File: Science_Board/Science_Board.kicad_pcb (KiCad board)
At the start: 2 copper layers, 217 x 149.5 mm, 141 parts, among them IC1 TCKE603RA, IC2 TCKE603RA, IC3 TCKE603RM, J1 Conn_01x02, J10 Conn_01x02, J11 Conn_01x03, J12 Conn_01x03, J13 Conn_01x03, J14 Conn_01x03, J15 Conn_01x03, J16 Conn_01x03, J17 Conn_01x03, J18 Conn_01x03, J19 Conn_01x02, J2 RJ45_LED_Shielded, J20 Molex_Megafit_02, J21 Molex_Megafit_02, J22 Molex_Megafit_02, J23 Conn_01x02, J3 Molex_Megafit_02, J4 Molex_Megafit_02, J5 Conn_01x05, J6 Conn_01x04, J7 Conn_01x03, J8 Conn_01x03, J9 Conn_01x02, Q1 BS250, Q2 NMOS, Q3 NMOS, Q4 NMOS, Q5 NMOS, SW1 SW_Push, SW10 SW_Push, SW11 SW_Push, SW12 SW_SPDT, SW2 SW_Push, SW3 SW_Push, SW4 SW_Push, SW5 SW_Push, SW6 SW_Push, SW7 SW_Push, SW8 SW_Push, SW9 SW_Push, U3 LM22678TJ-5, U5 PCA9685PW

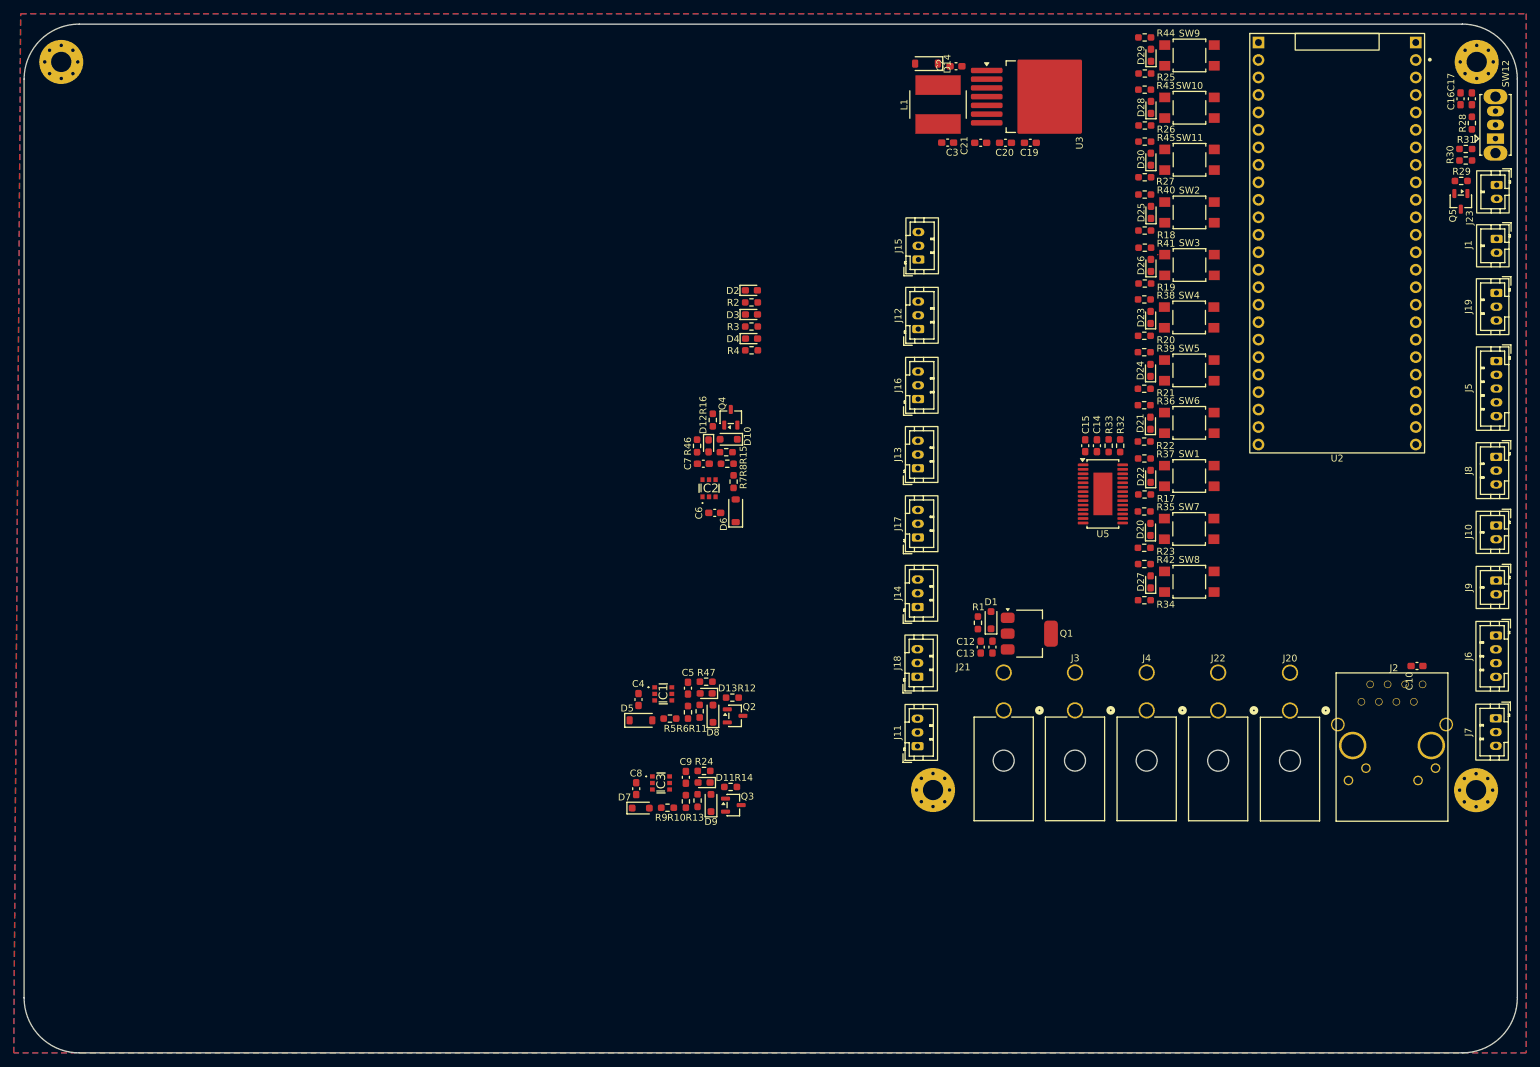
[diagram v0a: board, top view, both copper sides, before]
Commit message: Layout changes
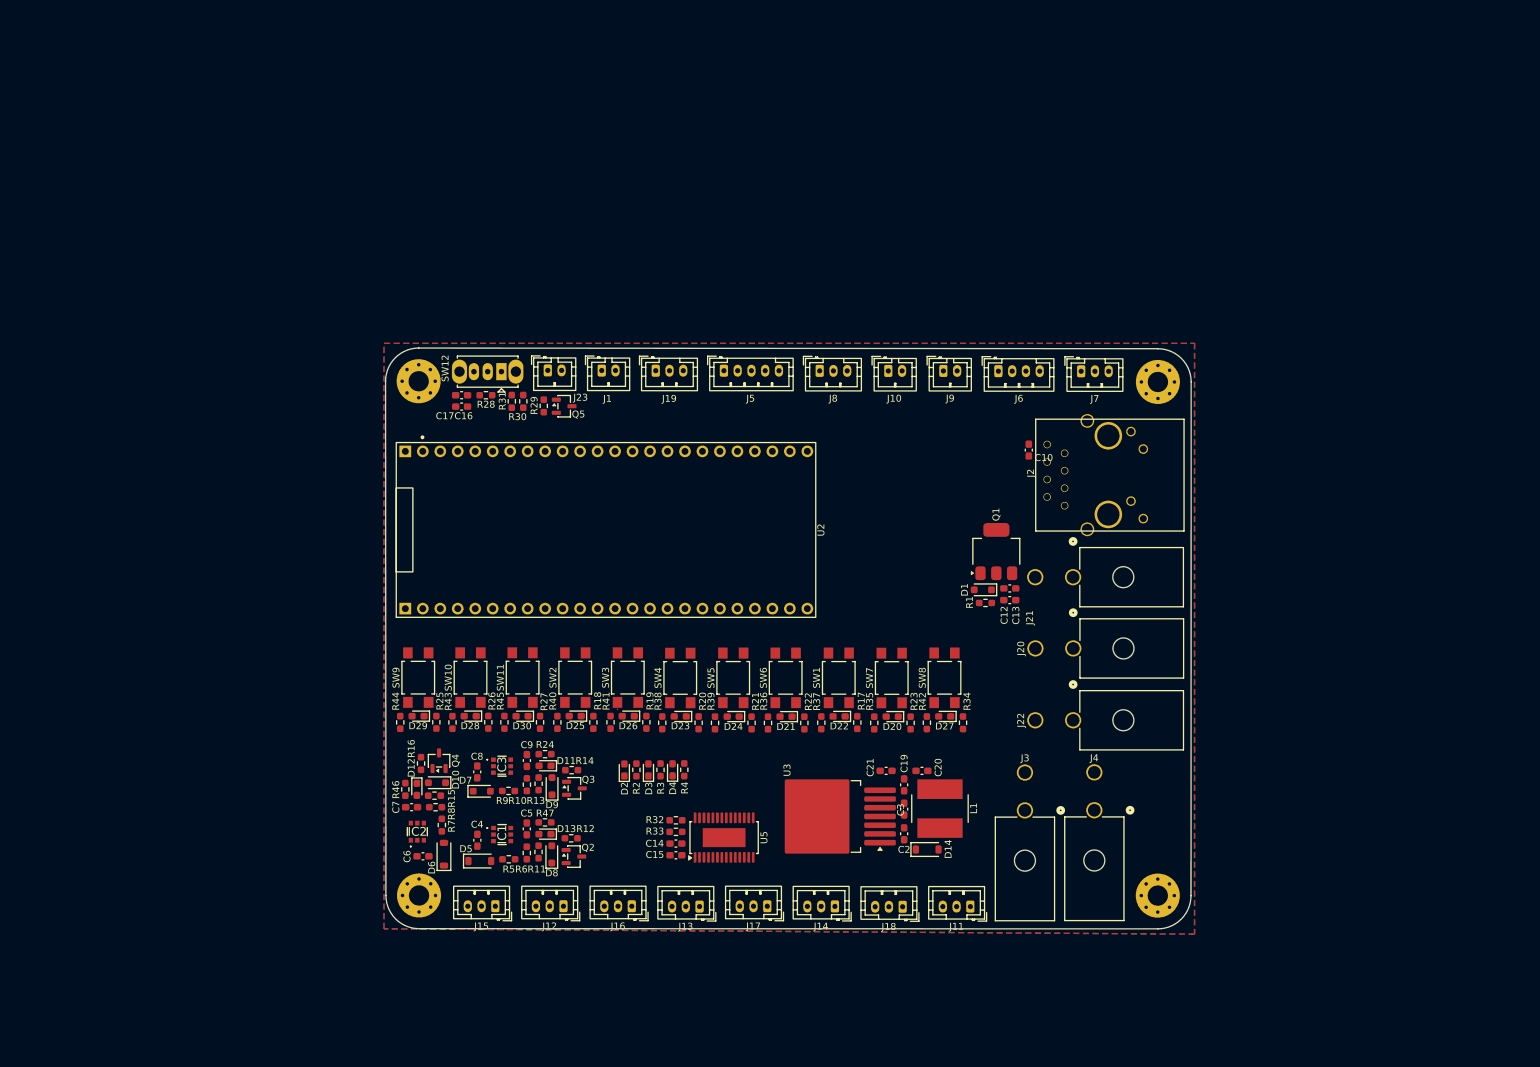
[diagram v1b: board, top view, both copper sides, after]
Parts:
- moved H2 160.6 mm to (87.8, 66.9), turned to 90 degrees
- moved C17 153.0 mm to (94.1, 68.9), turned to 0 degrees
- moved C16 151.9 mm to (94.1, 70.6), turned to 180 degrees
- moved U2 150.9 mm to (84.1, 101.7), turned to 90 degrees
- moved R28 148.6 mm to (97.6, 68.9), turned to 180 degrees
- moved SW12 148.4 mm to (99.9, 65.5), turned to 180 degrees
- moved R44 147.0 mm to (85.2, 116.5), turned to 90 degrees
- moved SW9 144.0 mm to (87.8, 110.0), turned to 90 degrees
- moved D29 143.4 mm to (87.8, 115.6), turned to 180 degrees
- moved R31 143.4 mm to (101.4, 69.8), turned to 90 degrees
- moved R30 141.4 mm to (103.0, 69.8), turned to 90 degrees
- moved J23 140.5 mm to (106.6, 65.3), turned to 0 degrees
- moved R25 139.6 mm to (90.4, 116.5), turned to 90 degrees
- moved R29 137.3 mm to (106.0, 70.5), turned to 90 degrees
- moved R43 136.3 mm to (92.8, 116.5), turned to 90 degrees
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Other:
- board size 217 x 149.5 mm -> 117.1 x 84.4 mm

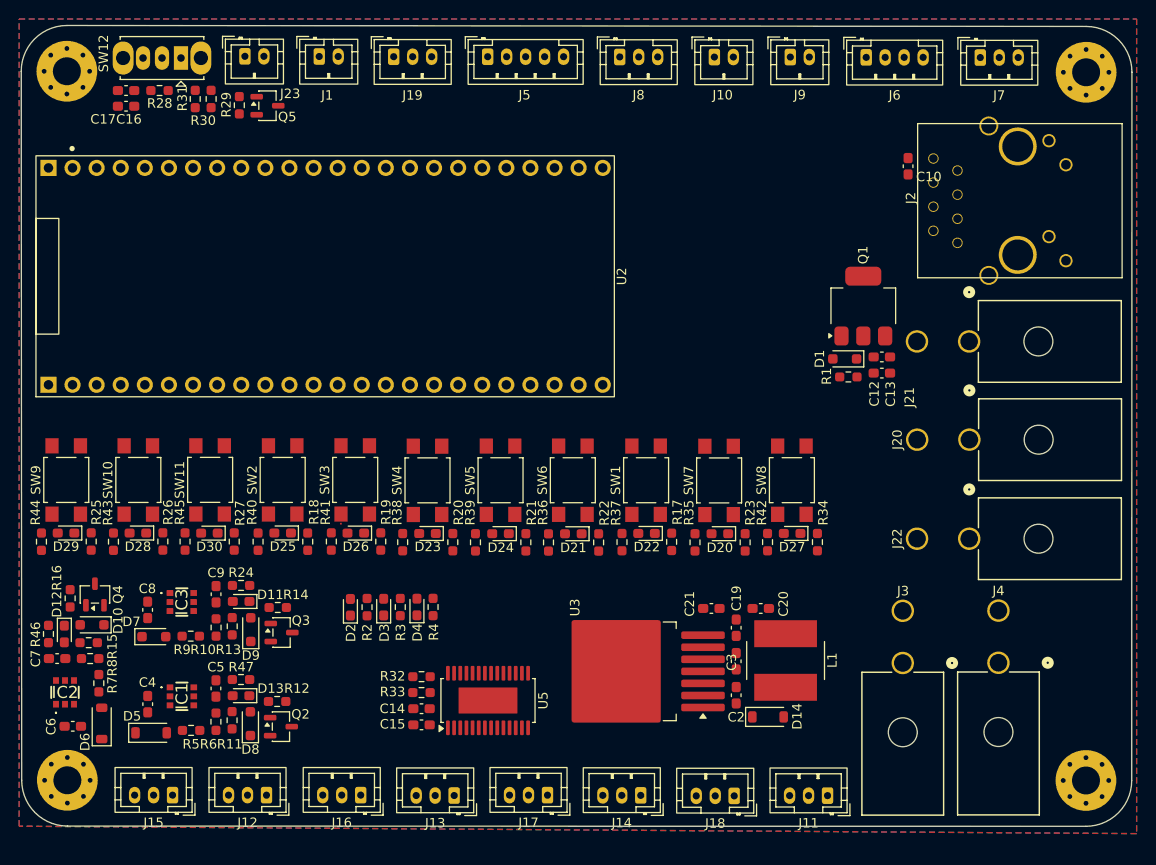
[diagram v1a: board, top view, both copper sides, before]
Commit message: layout look better
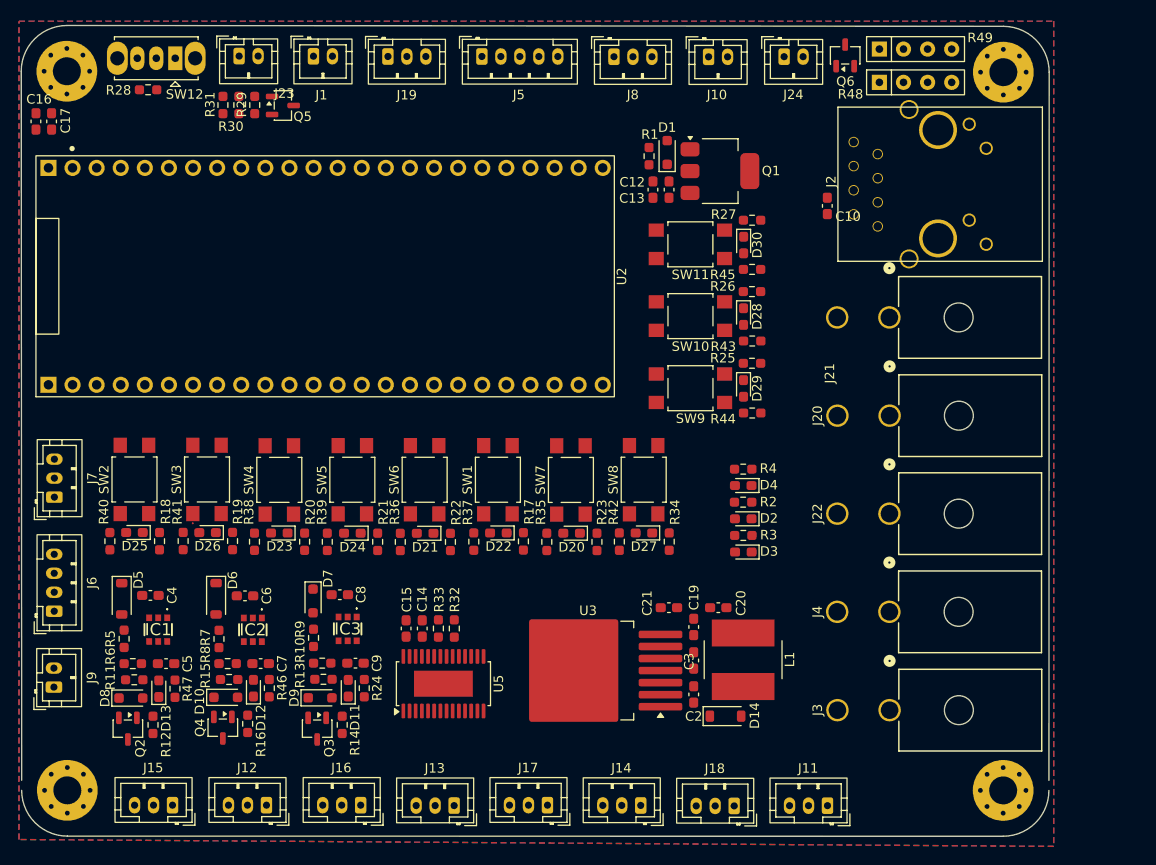
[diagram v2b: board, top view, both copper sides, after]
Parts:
- added J24: Conn_01x02, Connector_JST:JST_PH_B2B-PH-K_1x02_P2.00mm_Vertical, F.Cu at (163.4, 65.4)
- added Q6: NMOS, Package_TO_SOT_SMD:SOT-23-3, F.Cu at (169.9, 65.2)
- added R48: 100, Resistor_THT:R_Array_SIP4, F.Cu at (173.5, 68.1)
- added R49: 10k, Resistor_THT:R_Array_SIP4, F.Cu at (173.5, 64.6)
- moved J7 108.0 mm to (86.5, 111.8), turned to 90 degrees
- moved J6 103.6 mm to (86.5, 123.8), turned to 90 degrees
- moved J9 102.1 mm to (86.5, 131.8), turned to 90 degrees
- moved R44 76.1 mm to (160.1, 102.9), turned to 180 degrees
- moved D29 73.0 mm to (159.2, 100.3), turned to -90 degrees
- moved R25 72.1 mm to (160.1, 97.7), turned to 180 degrees
- moved R43 70.6 mm to (160.1, 95.3), turned to 180 degrees
- moved D28 67.8 mm to (159.2, 92.8), turned to -90 degrees
- moved R26 67.4 mm to (160.1, 90.1), turned to 180 degrees
- moved SW9 66.5 mm to (153.6, 100.3), turned to 180 degrees
- moved R45 66.3 mm to (160.1, 87.8), turned to 180 degrees
- moved R27 64.2 mm to (160.1, 82.6), turned to 180 degrees
- moved D30 64.0 mm to (159.2, 85.2), turned to -90 degrees
- moved SW10 60.7 mm to (153.6, 92.7), turned to 180 degrees
- moved SW11 56.4 mm to (153.6, 85.1), turned to 180 degrees
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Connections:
- J20 pad 1: +PV -> +Vpre
- J21 pad 1: Net-(J21-Pad1) -> +Vpre
- J3 pad 1: +PV -> +Vpre
- J4 pad 1: +PV -> +Vpre
- Q1 pad 2: Net-(J21-Pad1) -> +Vpre
- Q1 pad 4: Net-(J21-Pad1) -> +Vpre
- U2 pad 42: unconnected-(U2-PB0-Pad42) -> TEMP_CONTROL
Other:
- board size 117.1 x 84.4 mm -> 108.3 x 85.5 mm
